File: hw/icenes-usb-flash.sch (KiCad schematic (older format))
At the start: 29 parts, among them U4 iCE40HX8K-CT256, U5 93LC56C-I_SN, U6 FT2232H, U7 AT25SF041-SSHD, X1 DSC1001DI2-012.0000

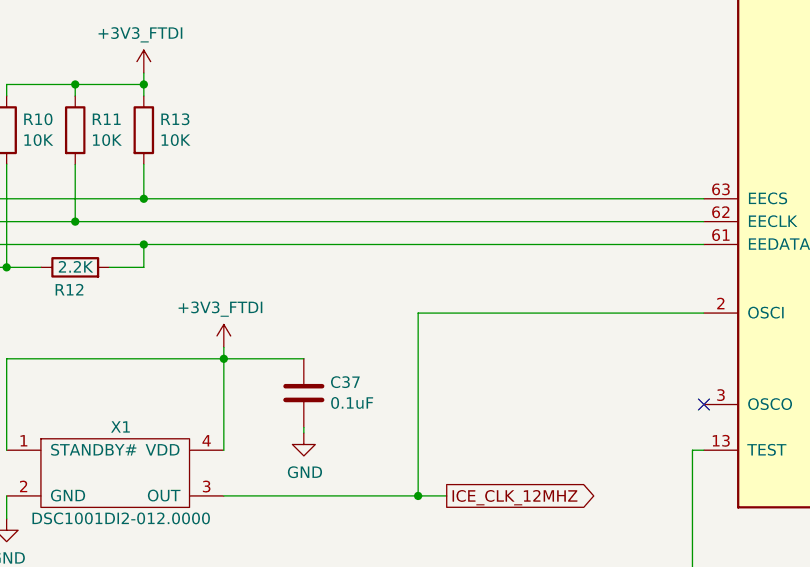
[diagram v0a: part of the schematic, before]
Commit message: Rough board layout.
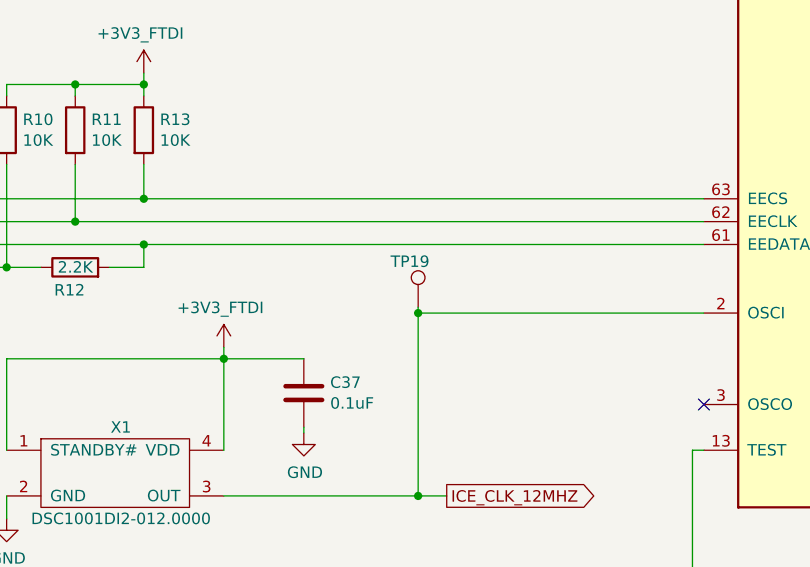
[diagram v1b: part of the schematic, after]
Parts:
- added TP19: TestPoint, TestPoint:TestPoint_Pad_D1.0mm, symbol icenes-library:TestPoint
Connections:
- net ICE_CLK_12MHZ: now also TP19.1
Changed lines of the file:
@@
 Text Label 12275 2650 2    50   ~ 0
 iCE_SS_B
+$Comp
+L icenes-library:TestPoint TP19
+U 1 1 5DE04EAE
+P 4450 6325
+F 0 "TP19" H 4500 6525 50  0000 R CNN
+F 1 "TestPoint" H 4450 6525 50  0001 C CNN
+F 2 "TestPoint:TestPoint_Pad_D1.0mm" H 4650 6325 50  0001 C CNN
+F 3 "~" H 4650 6325 50  0001 C CNN
+	1    4450 6325
+	1    0    0    -1
+$EndComp
+Wire Wire Line
+	4450 6325 4450 6350
+Connection ~ 4450 6350
 $EndSCHEMATC

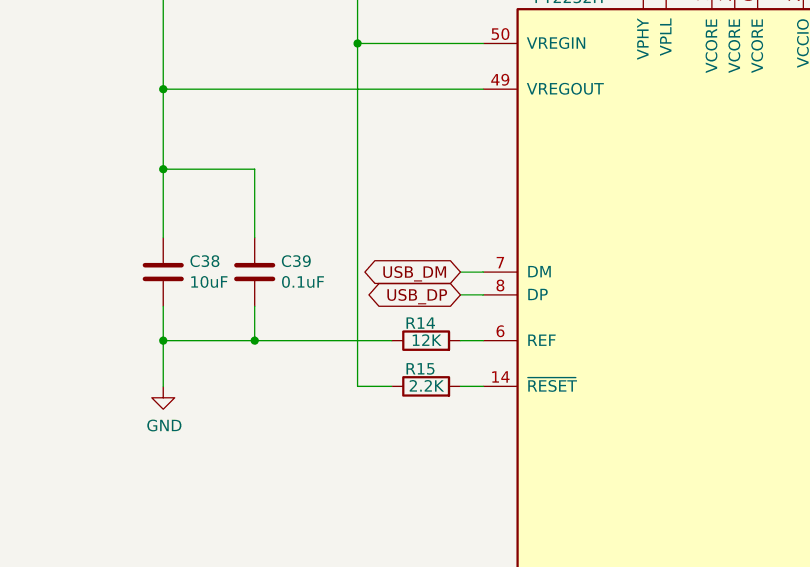
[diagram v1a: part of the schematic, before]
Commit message: Layout.
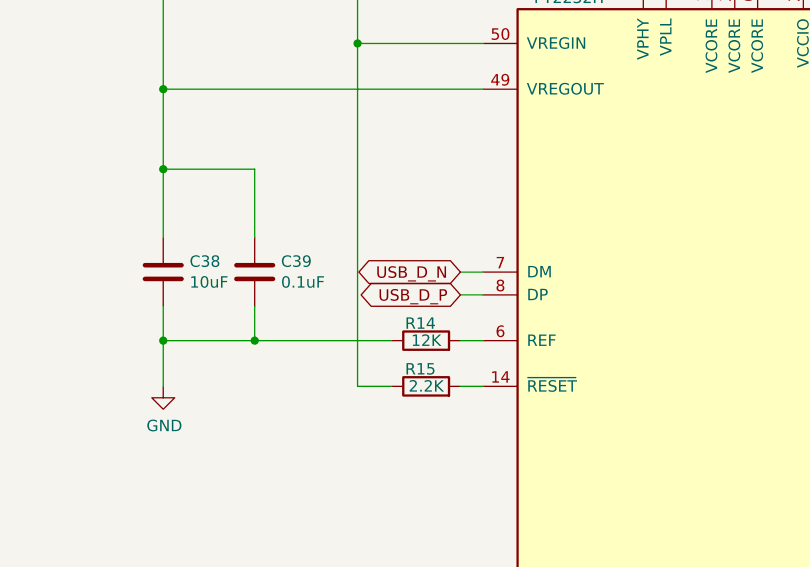
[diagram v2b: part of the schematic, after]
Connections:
- net USB_DM renamed USB_D_N
- net USB_DP renamed USB_D_P
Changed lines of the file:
@@
 $EndComp
 Text GLabel 5600 4250 0    50   BiDi ~ 0
-USB_DM
+USB_D_N
 Text GLabel 5600 4350 0    50   BiDi ~ 0
-USB_DP
+USB_D_P
 Text GLabel 8550 3850 2    50   BiDi ~ 0
 iCE_DONE

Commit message: Layout. Cleaned up nes connector footprints. Adjusted LED (D1) series resistor. Adjusted the voltage divider to BCBUS7 on FT2232H. Set pull up resistor to CDONE to 10k.
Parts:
- R16: value R4.7K -> R6.04k; symbol icenes-library:R4.7K -> icenes-library:R6.04k; Part number RC0603FR-072K2L -> RC0603FR-076K04L; Resistance 4.7K -> 6.04k
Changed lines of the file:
@@
 $EndComp
 $Comp
-L icenes-library:R4.7K R16
+L icenes-library:R6.04k R16
 U 1 1 5D99454A
 P 8750 6475
 F 0 "R16" V 8704 6545 50  0000 L CNN
-F 1 "R4.7K" H 8750 6375 50  0001 C CNN
+F 1 "R6.04k" H 8750 6375 50  0001 C CNN
 F 2 "Resistor_SMD:R_0603_1608Metric_Pad1.05x0.95mm_HandSolder" V 8750 6475 50  0001 C CNN
 F 3 "https://www.mouser.se/datasheet/2/447/PYu-RC_Group_51_RoHS_L_10-1527934.pdf" V 8750 6475 50  0001 C CNN
-F 4 "4.7K" V 8795 6545 50  0000 L CNN "Resistance"
+F 4 "6.04k" V 8795 6545 50  0000 L CNN "Resistance"
 F 5 "Yageo" H 8750 6475 50  0001 C CNN "Manufacturer"
-F 6 "RC0603FR-072K2L" H 8750 6475 50  0001 C CNN "Part number"
+F 6 "RC0603FR-076K04L" H 8750 6475 50  0001 C CNN "Part number"
 	1    8750 6475
 	0    1    1    0
